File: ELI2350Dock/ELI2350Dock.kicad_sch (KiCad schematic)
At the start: 13 parts, among them J1 Conn_01x32_Pin, J2 Conn_01x32_Pin

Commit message: doc pre-reroute
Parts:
- CN2: footprint emutelab:CONN-SMD_HC-PBB23L-60DP-0.5V8-G2-01 -> emutelab:CONN-SMD_HC-PBB23L-60DP-0.5V10-G2-01
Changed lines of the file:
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@@
 			)
 		)
-		(property "Footprint" "emutelab:CONN-SMD_HC-PBB23L-60DP-0.5V8-G2-01"
+		(property "Footprint" "emutelab:CONN-SMD_HC-PBB23L-60DP-0.5V10-G2-01"
 			(at 62.23 67.31 0)
 			(effects

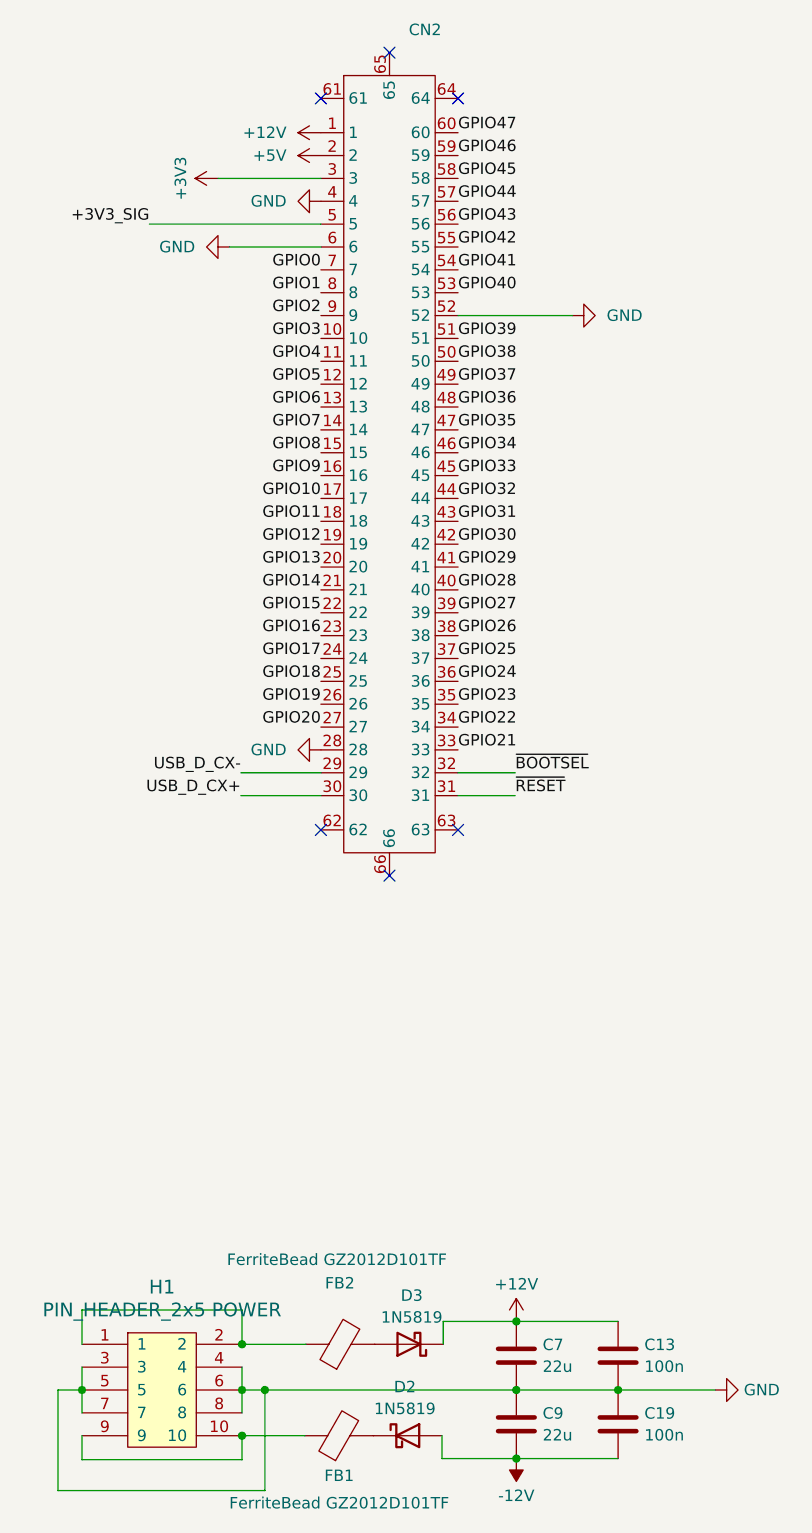
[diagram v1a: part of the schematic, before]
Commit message: bboard
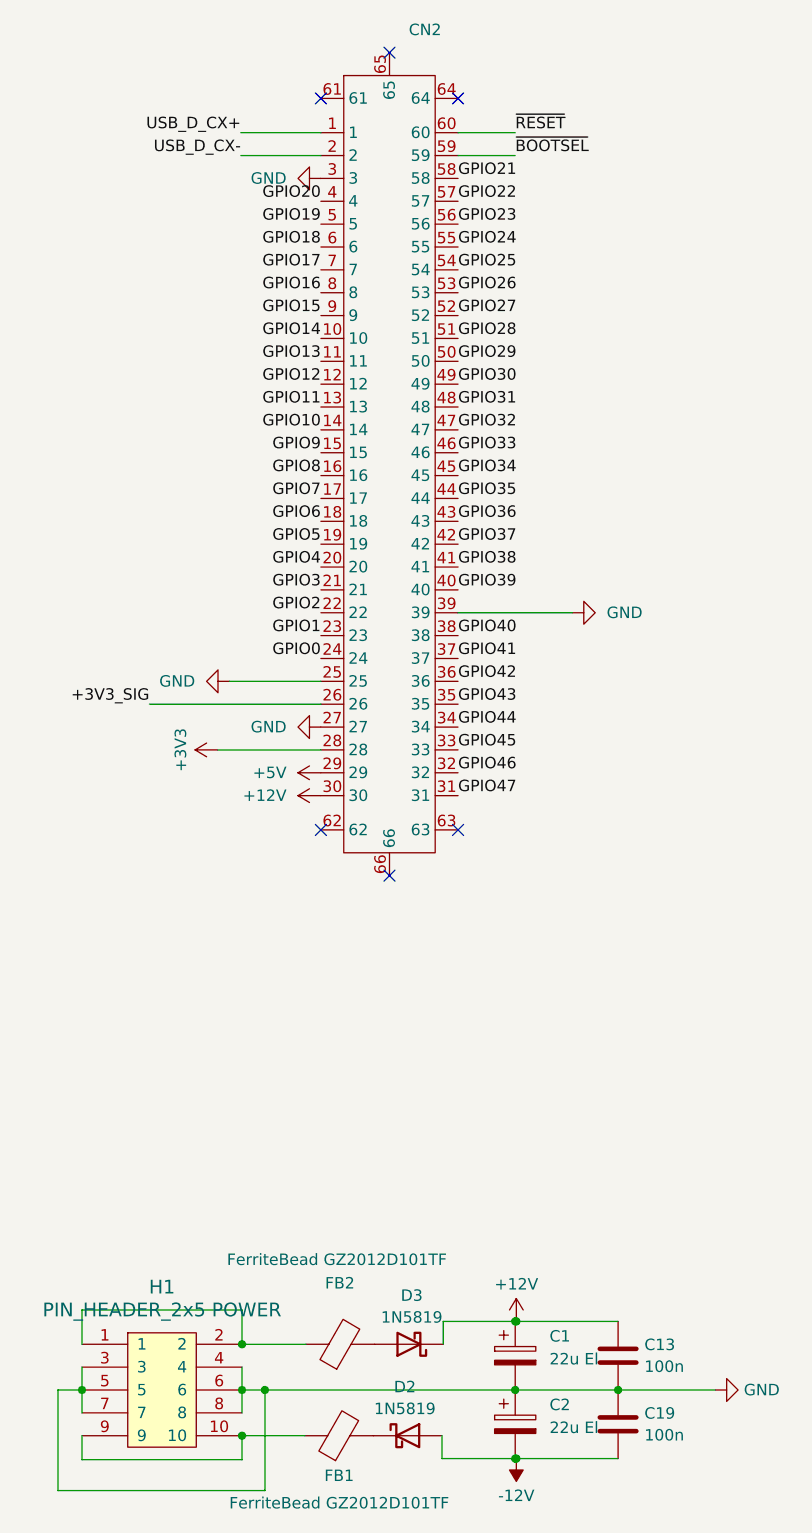
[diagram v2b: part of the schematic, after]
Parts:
- removed C7, C9: 22u, Capacitor_SMD:C_0805_2012Metric, symbol Device:C
- added C1, C2: 22u El, Capacitor_SMD:CP_Elec_4x3.9, symbol Device:C_Polarized
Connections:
- net +12V: now also CN2.30, C1.1; no longer CN2.1
- net +3V3: now also CN2.28; no longer CN2.3
- net +3V3_SIG: now also CN2.26; no longer CN2.5
- net +5V: now also CN2.29; no longer CN2.2
- net -12V: now also C2.2
- net GND: now also CN2.25, CN2.27, CN2.3, CN2.39, C1.2, C2.1; no longer CN2.28, CN2.4, CN2.52, CN2.6
- net GPIO0: now also CN2.24; no longer CN2.7
- net GPIO1: now also CN2.23; no longer CN2.8
- net GPIO10: now also CN2.14; no longer CN2.17
- net GPIO11: now also CN2.13; no longer CN2.18
- net GPIO12: now also CN2.12; no longer CN2.19
- net GPIO13: now also CN2.11; no longer CN2.20
- net GPIO14: now also CN2.10; no longer CN2.21
- net GPIO15: now also CN2.9; no longer CN2.22
- net GPIO16: now also CN2.8; no longer CN2.23
- net GPIO17: now also CN2.7; no longer CN2.24
- net GPIO18: now also CN2.6; no longer CN2.25
- net GPIO19: now also CN2.5; no longer CN2.26
- net GPIO2: now also CN2.22; no longer CN2.9
- net GPIO20: now also CN2.4; no longer CN2.27
- net GPIO21: now also CN2.58; no longer CN2.33
- net GPIO22: now also CN2.57; no longer CN2.34
- net GPIO23: now also CN2.56; no longer CN2.35
- net GPIO24: now also CN2.55; no longer CN2.36
- net GPIO25: now also CN2.54; no longer CN2.37
- net GPIO26: now also CN2.53; no longer CN2.38
- net GPIO27: now also CN2.52; no longer CN2.39
- net GPIO28: now also CN2.51; no longer CN2.40
- net GPIO29: now also CN2.50; no longer CN2.41
- net GPIO3: now also CN2.21; no longer CN2.10
- net GPIO30: now also CN2.49; no longer CN2.42
- net GPIO31: now also CN2.48; no longer CN2.43
- net GPIO32: now also CN2.47; no longer CN2.44
- net GPIO33: now also CN2.46; no longer CN2.45
- net GPIO34: now also CN2.45; no longer CN2.46
- net GPIO35: now also CN2.44; no longer CN2.47
- net GPIO36: now also CN2.43; no longer CN2.48
- net GPIO37: now also CN2.42; no longer CN2.49
- net GPIO38: now also CN2.41; no longer CN2.50
- net GPIO39: now also CN2.40; no longer CN2.51
- net GPIO4: now also CN2.20; no longer CN2.11
- net GPIO40: now also CN2.38; no longer CN2.53
- net GPIO41: now also CN2.37; no longer CN2.54
- net GPIO42: now also CN2.36; no longer CN2.55
- net GPIO43: now also CN2.35; no longer CN2.56
- net GPIO44: now also CN2.34; no longer CN2.57
- net GPIO45: now also CN2.33; no longer CN2.58
- net GPIO46: now also CN2.32; no longer CN2.59
- net GPIO47: now also CN2.31; no longer CN2.60
- net GPIO5: now also CN2.19; no longer CN2.12
- net GPIO6: now also CN2.18; no longer CN2.13
- net GPIO7: now also CN2.17; no longer CN2.14
- net GPIO8: now also CN2.16; no longer CN2.15
- net GPIO9: now also CN2.15; no longer CN2.16
- net USB_D_CX+: now also CN2.1; no longer CN2.30
- net USB_D_CX-: now also CN2.2; no longer CN2.29
- net ~{BOOTSEL}: now also CN2.59; no longer CN2.32
- net ~{RESET}: now also CN2.60; no longer CN2.31
